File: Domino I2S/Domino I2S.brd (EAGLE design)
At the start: 33.9 x 33 mm, 58 parts, among them J1 MH4-1, J2 MIC-45-22, J3 MH4-1, J4 MH2-1, J5 MH4-1, J6 DLT1120A, J7 MH4-1, J8 MH2-1, U1 WM8978CGEFL

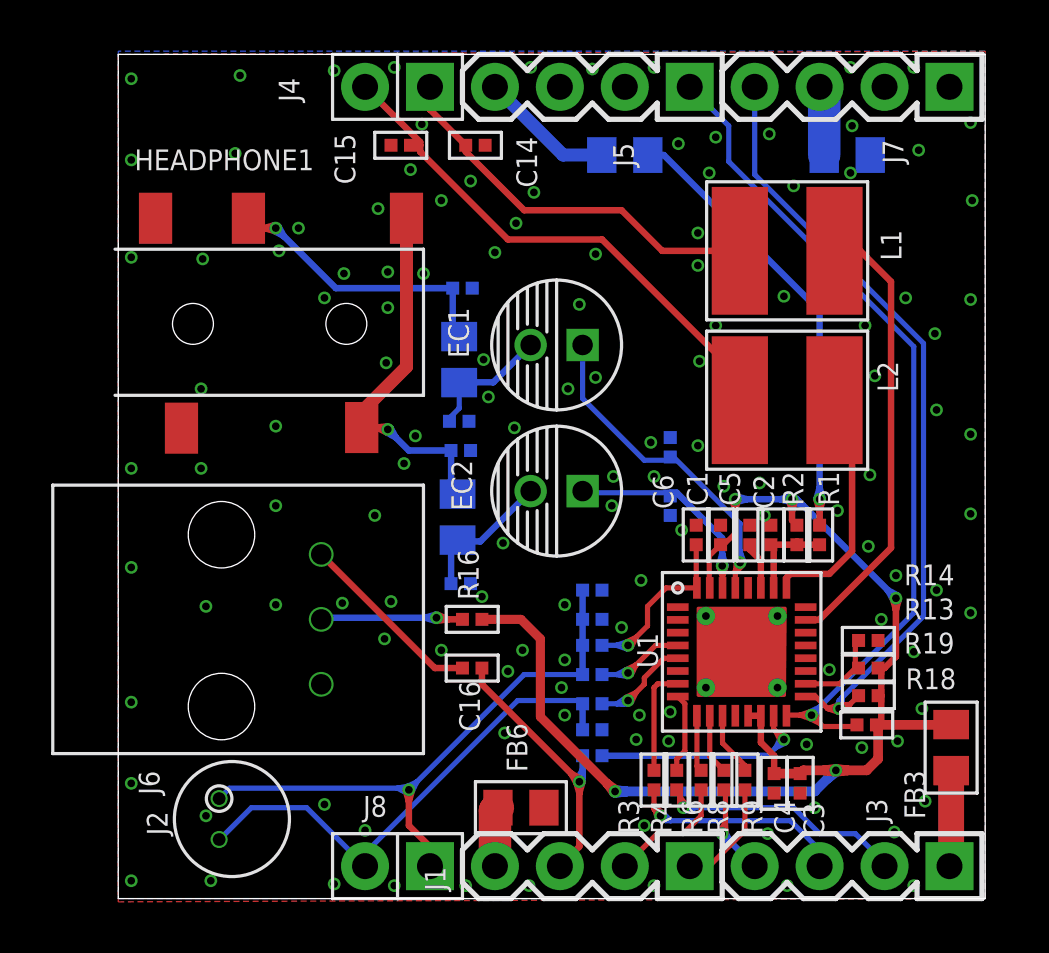
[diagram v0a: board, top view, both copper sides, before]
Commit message: Domino I2S Rev. A: added mounting hole and silkscreen artwork
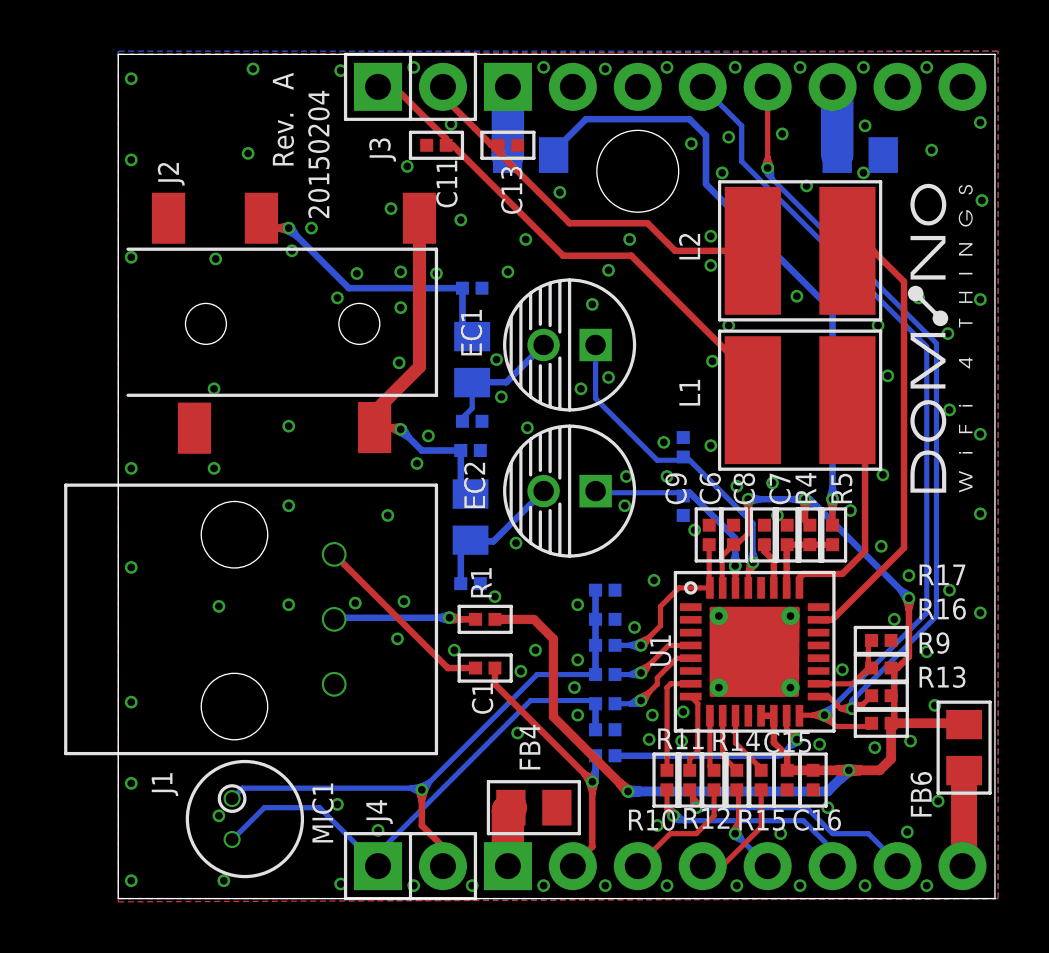
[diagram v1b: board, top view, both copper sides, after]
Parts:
- removed HEADPHONE1: ST-3538-050, Domino:ST-3538-050
- removed J7: MH4-1, Domino:MH4-1-0.1
- removed J8: MH2-1, Domino:MH2-1-0.1
- removed R19: 10k, Domino:R0402
- added MIC1: MIC-45-22, Domino:MIC-45-22
- added R15: 22R, Domino:R0402
- added U$12, U$14: (no value), Domino:DOMINO_LOGO_SMALL
- added U$13: (no value), Domino:CE_LOGO_SMALL
- added U$15: (no value), Domino:ESD_LOGO
- added U$16: (no value), Domino:FCC_LOGO_SMALL
- added U$17: (no value), Domino:OPEN_HARDWARE_LOGO
- added U$18: (no value), Domino:RECYCLE_BIN_LOGO
- added U$19: (no value), Domino:ROHS_LOGO
- C1: value 4u7 -> 1u
- C10: value 1n -> 220p
- C11: value 1n -> 10n
- C12: value 33p -> 1u
- C13: value 1u -> 10n
- C14: value 10n -> 1u
- C15: value 10n -> 4u7
- C16, C9: value 1u -> 4u7
- C2, C3: value 4u7 -> 33p
- C4, C5: value 4u7 -> 1n
- C7: value 220p -> 4u7
- C8: value 33p -> 4u7
- J1: value MH4-1 -> DLT1120A; device Domino:MH4-1-0.1 -> Domino:DLT1120A
- J2: value MIC-45-22 -> ST-3538-050; device Domino:MIC-45-22 -> Domino:ST-3538-050
- J3: value MH4-1 -> MH2-1; device Domino:MH4-1-0.1 -> Domino:MH2-1-0.1
- J5: value MH4-1 -> MH8-1; device Domino:MH4-1-0.1 -> Domino:MH8-1-0.1
- J6: value DLT1120A -> MH8-1; device Domino:DLT1120A -> Domino:MH8-1-0.1
- R10: value 0R -> 22R
- R11, R12: value 4k7 -> 22R
- R14: value 10k -> 22R
- R16, R17: value 0R -> 10k
- R18: value 10k -> 0R
- R2: value 0R -> 4k7
- R3: value 22R -> 4k7
- R4, R8: value 22R -> 0R
- R5: value 47k -> 0R
- R6: value 22R -> 680R
- R7: value 680R -> 47k
- R9: value 22R -> 10k
- moved J3 37.8 mm to (10.2, 31.8), turned to 0 degrees
- moved J4 30.5 mm to (10.2, 1.27), turned to 0 degrees
- moved C15 29.1 mm to (26.2, 4.64), turned to 270 degrees
- moved FB3 28.4 mm to (16.1, 29.1), flipped to the bottom, turned to 0 degrees
- moved FB4 25.8 mm to (16.3, 3.56), flipped to the top
- moved C14 22.4 mm to (19.1, 7.62), flipped to the bottom
- moved C13 22.1 mm to (15.2, 29.5), flipped to the top
- moved J2 19.4 mm to (3.43, 22.5), turned to 0 degrees
- moved C3 18.3 mm to (13.8, 17.5), flipped to the bottom, turned to 0 degrees
- moved FB6 17.5 mm to (33.1, 5.91), turned to 90 degrees
- moved J1 16.9 mm to (8.45, 10.9), turned to 90 degrees
- moved R11 16.7 mm to (22.4, 4.64), flipped to the top, turned to 90 degrees
- moved R16 16.1 mm to (29.8, 9.02), turned to 0 degrees
- moved C12 16.1 mm to (19.1, 8.76)
- moved R3 15.7 mm to (13.8, 18.7), flipped to the bottom, turned to 180 degrees
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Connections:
- net +3V3: now also C15.1, C16.1, C6.1, FB6.2, R1.1, R16.2, R4.1, R9.2; no longer C1.1, C3.1, C4.1, FB3.2, R16.1, R18.2, R19.2, R2.1
- net +5V: now also FB3.1, R5.1; no longer FB4.1, R1.1
- net ADCDAT: now also J6.3, R12.1; no longer J1.2, R6.1
- net BCLK: now also J6.7, R11.1; no longer J3.2, R4.1
- net CSB: now also R18.1; no longer R17.1
- net DACDAT: now also J6.5, R14.1; no longer J3.4, R8.1
- net GND: now also C13.2, C16.2, C3.1, C5.2, C7.1, C9.2, FB4.2, J1.1, J2.1, J2.5, R17.1, R2.2, R3.2, R7.1, R8.1; no longer C1.2, C12.1, C14.2, C3.2, C5.1, C7.2, FB6.2, HEADPHONE1.1, HEADPHONE1.5, J6.1, R10.1, R11.2, R12.2, R14.1, R5.1
- net LOUT1: now also C5.1; no longer C10.1
- net LOUT2: now also L1.1; no longer L2.1
- net LRCK: now also J6.6, R10.1; no longer J3.3, R3.1
- net MCLK: now also J6.4, R15.1; no longer J1.1, R9.1
- net MICBIAS: now also C9.1, R6.2; no longer C6.1, R7.2
- net MICN: now also C14.2, J4.1, MIC1.-, R8.2; no longer C13.2, J2.-, J8.2, R10.2
- net MICP: now also C10.1, C12.2, J4.2, MIC1.+, R6.1, R7.2; no longer C7.1, C9.2, J2.+, J8.1, R5.2, R7.1
- net MODE: now also R16.1, R17.2; no longer R13.1, R14.2
- net N$1: now also R10.2; no longer R3.2
- net N$10: now also FB4.1, J6.1; no longer FB6.1, J1.4
- net N$11: now also FB3.2, J5.1; no longer FB4.2, J5.4
- net N$12: now also R3.1; no longer R11.1
- net N$13: now also R2.1; no longer R12.1
- net N$14: now also FB6.1, J6.8; no longer FB3.1, J3.1
- net N$15: now also J5.6; no longer J7.3
- net N$16: now also C3.2, J2.3, J2.4; no longer C8.2, HEADPHONE1.3, HEADPHONE1.4
- net N$17: now also C2.2, J2.2; no longer C12.2, HEADPHONE1.2
- net N$2: now also R11.2; no longer R4.2
- net N$3: now also R12.2; no longer R6.2
- net N$4: now also R14.2; no longer R8.2
- net N$5: now also R15.2; no longer R9.2
- net N$6: now also C12.1; no longer C9.1
- net N$7: now also C14.1; no longer C13.1
- net N$8: now also C1.1, J1.3; no longer C16.1, J6.3
- net N$9: now also J1.2, R1.2; no longer J6.2, R16.2
- net ROUT1: now also C4.1; no longer C11.1
- net ROUT2: now also L2.1; no longer L1.1
- net SCLK: now also J5.4, R13.1; no longer J5.1, R18.1
- net SDIN: now also J5.5, R9.1; no longer J7.4, R19.1
- net SPDIF_OUT: now also C1.2, J6.2, R18.2; no longer C16.2, J1.3, R17.2
- net SPKL: now also C11.1, J3.1, L1.2; no longer C15.1, J4.2, L2.2
- net SPKR: now also C13.1, J3.2, L2.2; no longer C14.1, J4.1, L1.2
- net SPKVDD: now also C7.2, R4.2, R5.2; no longer C2.2, R1.2, R2.2
- net VMID: now also C8.2; no longer C5.2
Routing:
- net +5V: track 19.9 -> 26.7 mm
- net N$11: track 5.28 -> 2.67 mm
- net SDIN: track 34.3 -> 36.6 mm, vias 1 -> 2
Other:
- board size 33.9 x 33 mm -> 34.3 x 33 mm
- board text added: "+3V3"
- board text added: "+5V"
- board text added: ">DATE"
- board text added: "GDN"
- board text added: "GND"
- board text added: "I2S_CK"
- board text added: "I2S_MCK"
- board text added: "I2S_MICIN"
- board text added: "I2S_SD"
- board text added: "I2S_WS"
- board text added: "MICN"
- board text added: "MICP"
- board text added: "SCLK"
- board text added: "SDIN"
- board text added: "SPDIF OUT"
- board text added: "SPDIF_OUT"
- board text added: "SPKL"
- board text added: "SPKR"
